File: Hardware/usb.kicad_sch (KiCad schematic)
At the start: 8 parts, among them J2 USB_C_Receptacle_USB2.0

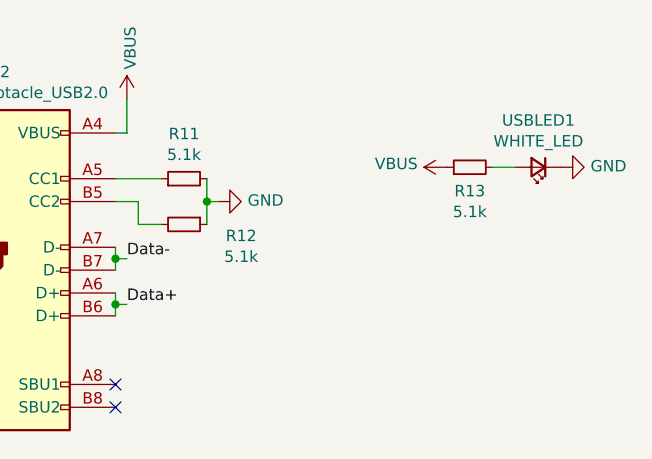
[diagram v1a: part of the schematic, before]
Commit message: layout
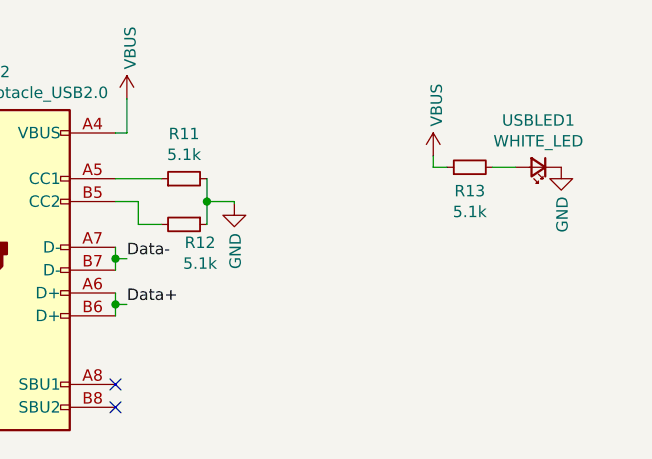
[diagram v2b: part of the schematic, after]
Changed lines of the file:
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@@
+	(wire
+		(pts
+			(xy 150.876 91.44) (xy 150.876 92.71)
+		)
+		(stroke
+			(width 0)
+			(type default)
+		)
+	)
 	(wire
 		(pts
@@
 	(wire
 		(pts
+			(xy 152.4 92.71) (xy 150.876 92.71)
+		)
+		(stroke
+			(width 0)
+			(type default)
+		)
+	)
+	(wire
+		(pts
 			(xy 125.73 99.06) (xy 125.73 96.52)
 		)
@@
 	(wire
 		(pts
-			(xy 125.73 96.52) (xy 127 96.52)
+			(xy 125.73 96.52) (xy 128.778 96.52)
 		)
 		(stroke
@@
 		(pts
 			(xy 118.11 99.06) (xy 120.65 99.06)
+		)
+		(stroke
+			(width 0)
+			(type default)
+		)
+	)
+	(wire
+		(pts
+			(xy 128.778 96.52) (xy 128.778 96.774)
 		)
 		(stroke
@@
 	(symbol
 		(lib_id "power:GND")
-		(at 127 96.52 90)
+		(at 128.778 96.774 0)
 		(unit 1)
 		(exclude_from_sim no)
@@
 		(dnp no)
 		(property "Reference" "#PWR031"
-			(at 133.35 96.52 0)
+			(at 128.778 103.124 0)
 			(effects
 				(font
@@
 		)
 		(property "Value" "GND"
-			(at 130.2512 96.393 90)
+			(at 128.905 100.0252 90)
 			(effects
 				(font
@@
 		)
 		(property "Footprint" ""
-			(at 127 96.52 0)
+			(at 128.778 96.774 0)
 			(effects
 				(font
@@
 		)
 		(property "Datasheet" ""
-			(at 127 96.52 0)
-			(effects
-				(font
-					(size 1.27 1.27)
-				)
-				(hide yes)
-			)
-		)
-		(property "Description" ""
-			(at 127 96.52 0)
+			(at 128.778 96.774 0)
+			(effects
+				(font
+					(size 1.27 1.27)
+				)
+				(hide yes)
+			)
+		)
+		(property "Description" ""
+			(at 128.778 96.774 0)
 			(effects
 				(font
@@
 		(dnp no)
 		(property "Reference" "R12"
-			(at 129.54 100.33 90)
+			(at 124.968 101.092 90)
 			(effects
 				(font
@@
 		)
 		(property "Value" "5.1k"
-			(at 129.54 102.6414 90)
+			(at 124.968 103.4034 90)
 			(effects
 				(font
@@
 	(symbol
 		(lib_id "power:GND")
-		(at 165.1 92.71 90)
+		(at 165.1 92.71 0)
 		(unit 1)
 		(exclude_from_sim no)
@@
 		(dnp no)
 		(property "Reference" "#PWR034"
-			(at 171.45 92.71 0)
+			(at 165.1 99.06 0)
 			(effects
 				(font
@@
 		)
 		(property "Value" "GND"
-			(at 168.3512 92.583 90)
+			(at 165.227 95.9612 90)
 			(effects
 				(font
@@
 	(symbol
 		(lib_id "power:VBUS")
-		(at 152.4 92.71 90)
+		(at 150.876 91.44 0)
 		(unit 1)
 		(exclude_from_sim no)
@@
 		(dnp no)
 		(property "Reference" "#PWR033"
-			(at 156.21 92.71 0)
+			(at 150.876 95.25 0)
 			(effects
 				(font
@@
 		)
 		(property "Value" "VBUS"
-			(at 149.1488 92.329 90)
+			(at 151.257 88.1888 90)
 			(effects
 				(font
@@
 		)
 		(property "Footprint" ""
-			(at 152.4 92.71 0)
+			(at 150.876 91.44 0)
 			(effects
 				(font
@@
 		)
 		(property "Datasheet" ""
-			(at 152.4 92.71 0)
-			(effects
-				(font
-					(size 1.27 1.27)
-				)
-				(hide yes)
-			)
-		)
-		(property "Description" ""
-			(at 152.4 92.71 0)
-			(effects
-				(font
+			(at 150.876 91.44 0)
+			(effects
+				(font
+					(size 1.27 1.27)
+				)
+				(hide yes)
+			)
+		)
+		(property "Description" ""
+			(at 150.876 91.44 0)
+			(effects
+				(font
